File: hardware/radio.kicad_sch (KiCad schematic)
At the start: 61 parts, among them J1 105450-0101, J2 Conn_01x02, J3 Conn_01x02, J4 Conn_01x04, J5 Conn_01x02_Male, Q1 Q_PMOS_DGS, Q2 Q_NMOS_DGS, Q3 Q_NMOS_DGS, Q4 Q_PMOS_DGS, SW1 SW_BOOT, SW2 SW_RST, SW3 SW_1, SW4 Rot_Enc, SW5 SW_2, SW6 SW_3, SW7 SW_PWR, U1 TP4056, U2 ESP32-WROOM-32, U3 TPS5432, U4 MAX98357

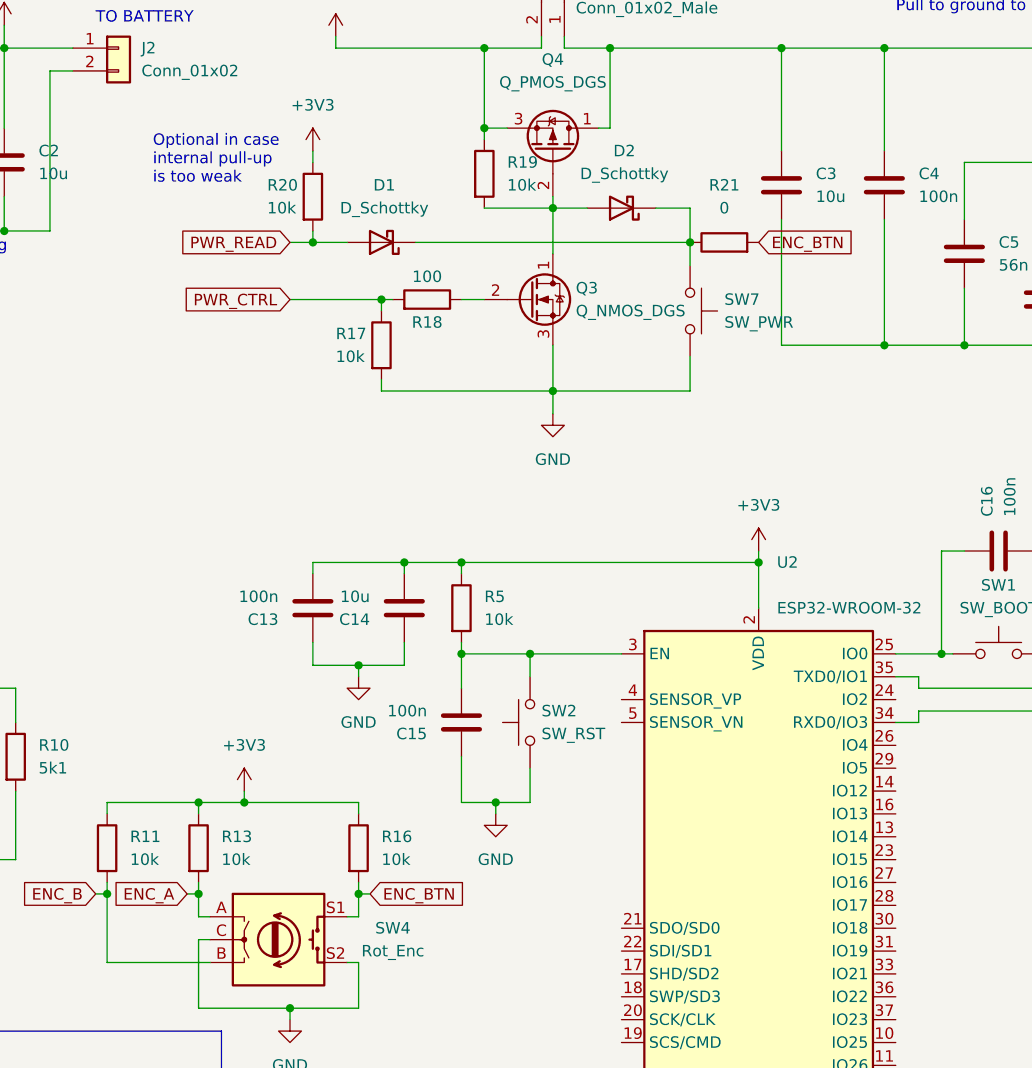
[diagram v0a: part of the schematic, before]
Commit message: placement
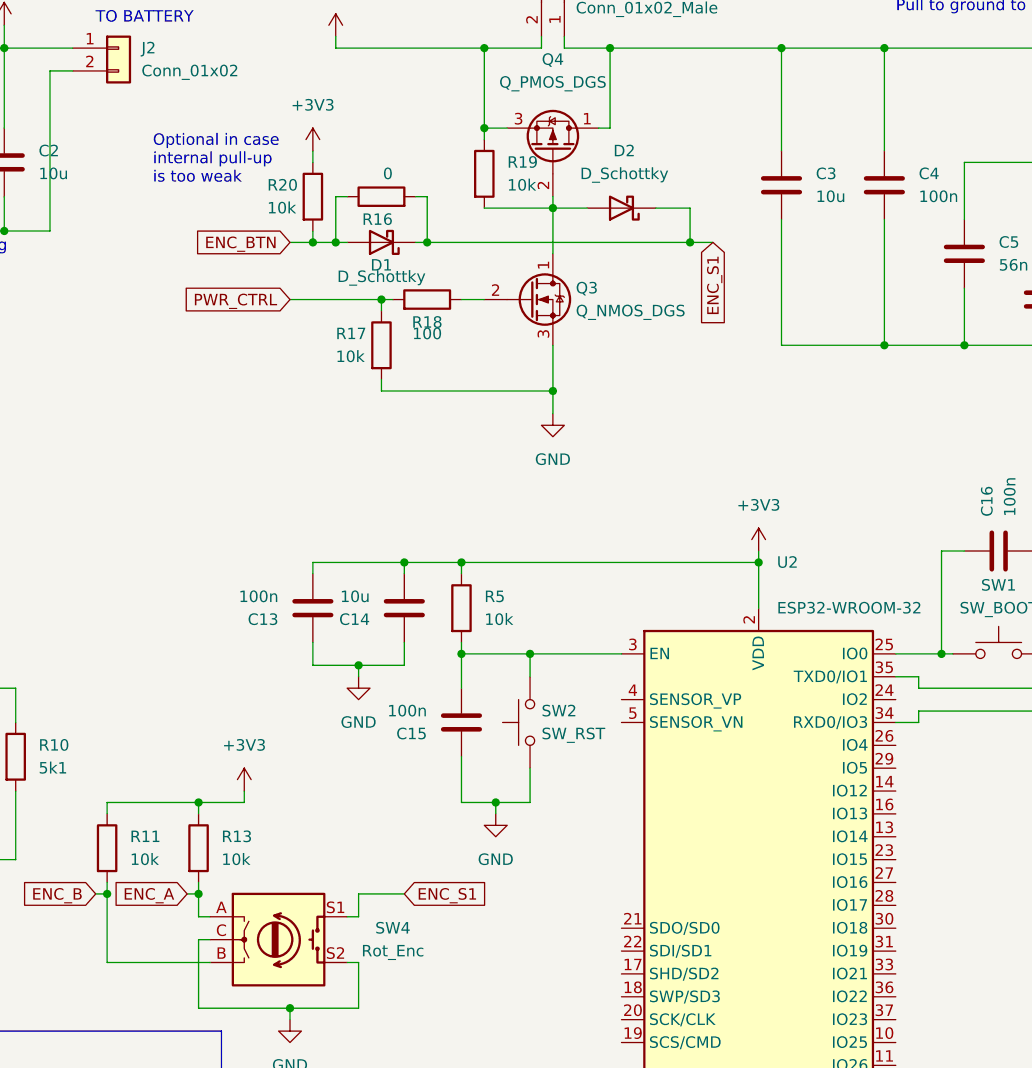
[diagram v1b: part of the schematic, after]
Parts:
- removed R21: 0, Resistor_SMD:R_0603_1608Metric, symbol Device:R
- removed SW7: SW_PWR, Button_Switch_SMD:SW_Push_1P1T_NO_6x6mm_H9.5mm, symbol Switch:SW_Push
- R16: value 10k -> 0
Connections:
- net PWR_READ is gone; now on net ENC_BTN: D1.2 (A), R20.2
- net +3V3: no longer R16.1
- net ENC_BTN: now also R16.1; no longer R16.2, SW4.S1
- net ENC_S1: now reaches D1.1 (K), D2.1 (K)
- net ENC_S1: now also R16.2, SW4.S1
